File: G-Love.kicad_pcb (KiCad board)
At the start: 2 copper layers, 130.4 x 73.5 mm, 154 parts, among them J4 XLR5_Ground, U14 TPS2113APWR, U18 MAX485E, Y1 16MHz, Y2 16MHz

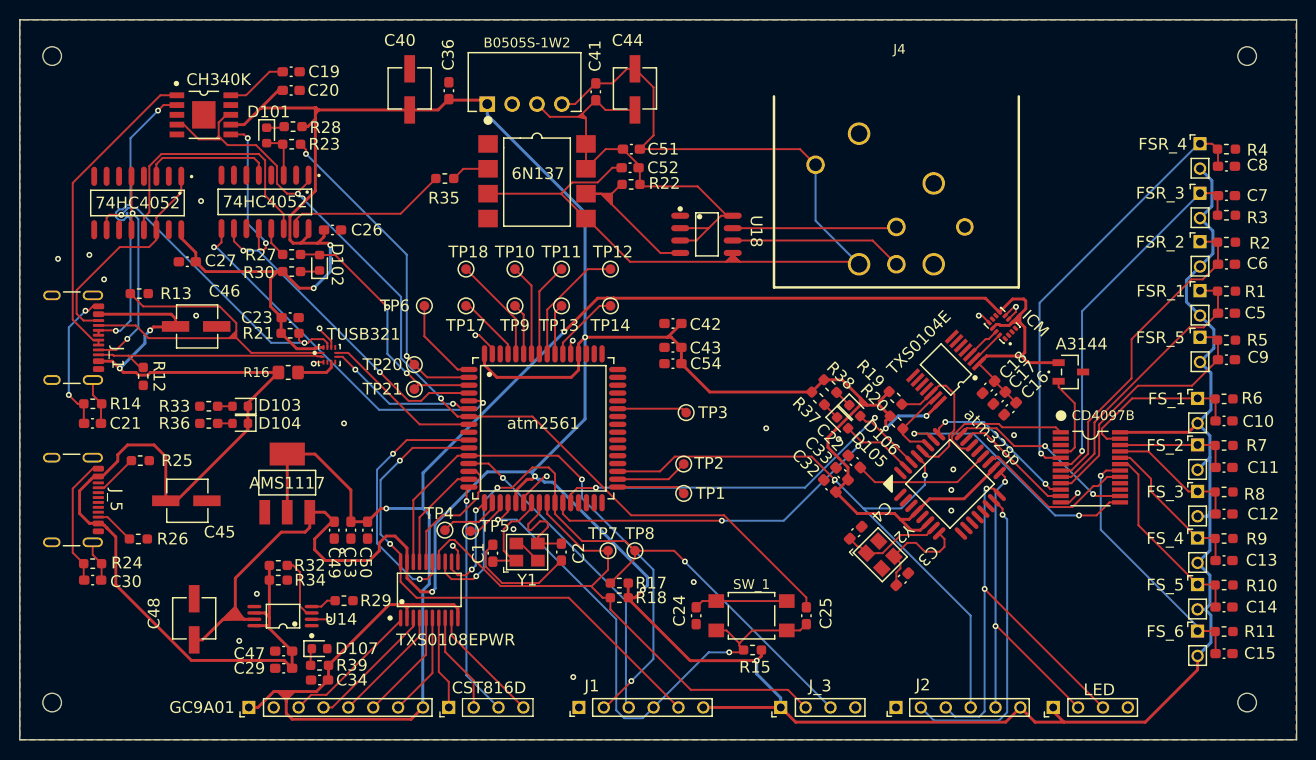
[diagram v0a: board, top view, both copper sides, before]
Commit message: fix routing and carrefour
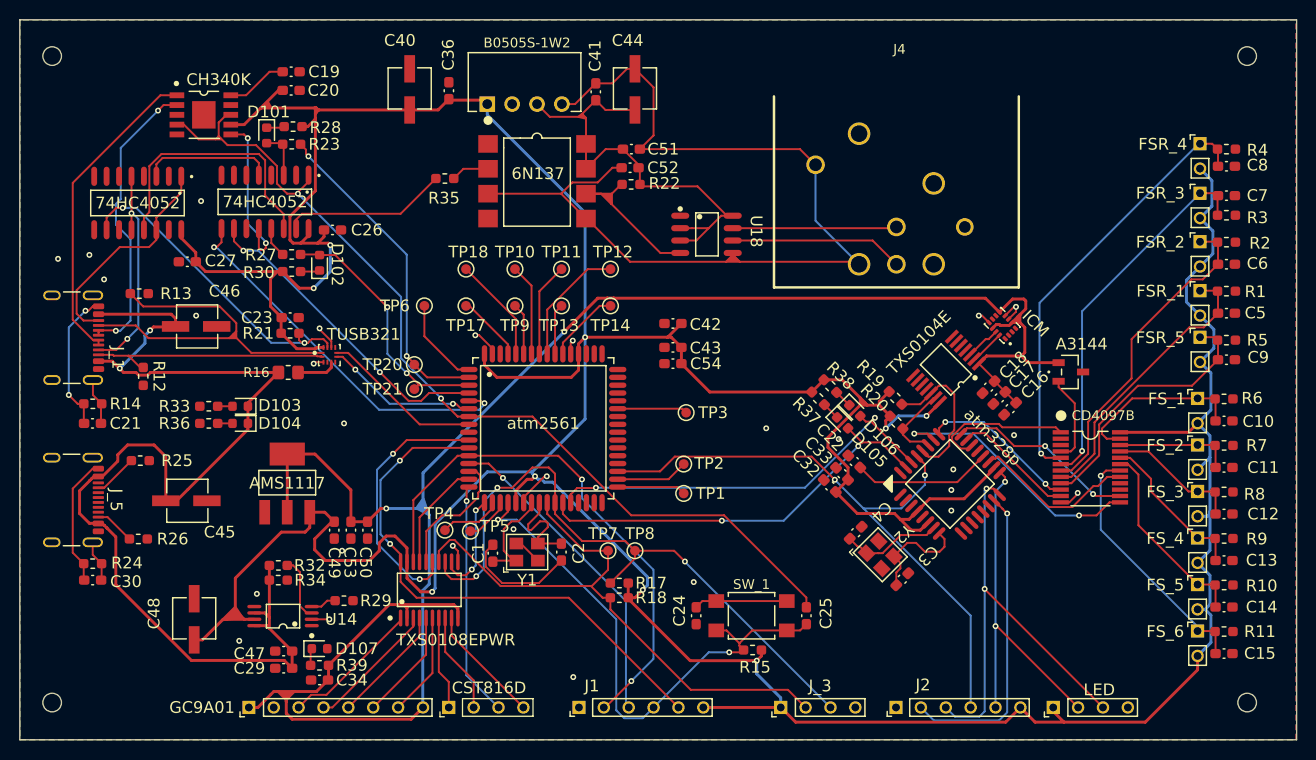
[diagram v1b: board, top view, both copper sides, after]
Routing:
- net /Data/power I/O/Data/UD-: track 32.2 -> 30.0 mm
